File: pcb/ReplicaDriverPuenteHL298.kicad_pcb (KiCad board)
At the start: 2 copper layers, 50 x 50 mm, 29 parts, among them J1 Conn_01x04, J2 Conn_01x02, J3 Conn_01x02, J4 Conn_01x02, J5 Conn_01x02, J6 Conn_01x02, J7 Conn_01x03, U1 L298HN, U2 LM78M05

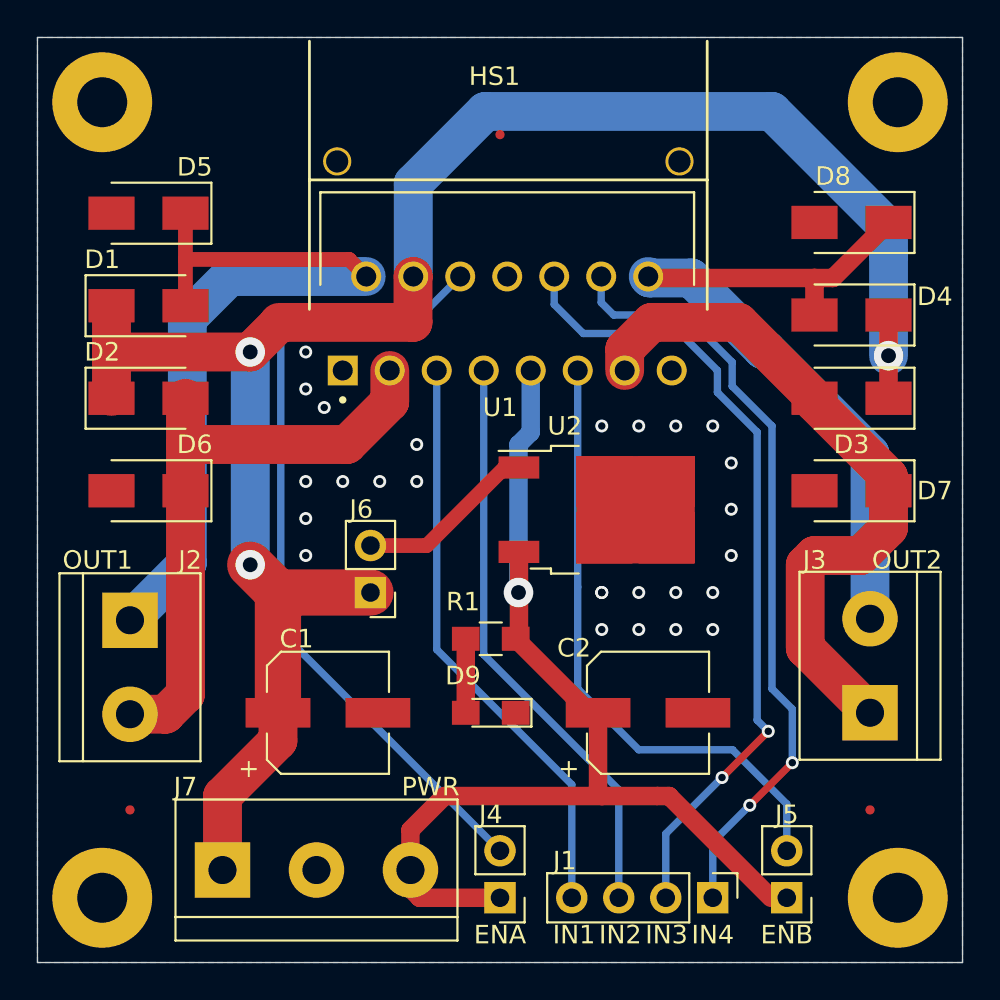
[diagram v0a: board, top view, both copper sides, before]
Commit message: Add files via upload
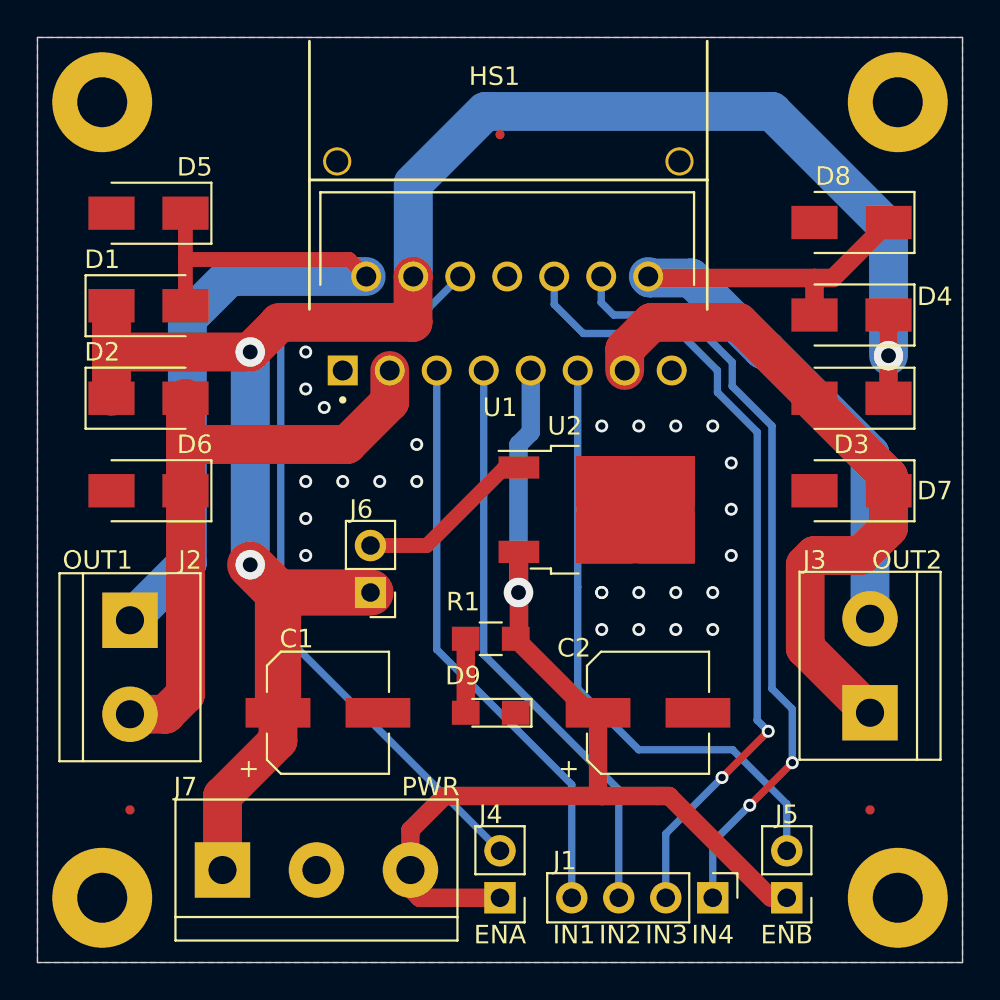
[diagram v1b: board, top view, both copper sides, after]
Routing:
- added copper zone on F.Cu, net GND
